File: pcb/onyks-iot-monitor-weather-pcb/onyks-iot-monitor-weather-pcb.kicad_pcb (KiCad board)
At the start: 2 copper layers, 100 x 100 mm, 25 parts, among them J1 53398-0371, J10 Conn_01x02_Pin, J2 53398-0371, J3 53048-0810, J4 53398-0371, J5 53398-0371, J6 53398-0371, J7 53398-0371, J8 53398-0371, J9 53398-0371, Q1 SS8050, Q2 SS8050, U1 ESP32-WROOM-32D, U2 AMS1117, U6 BMP280

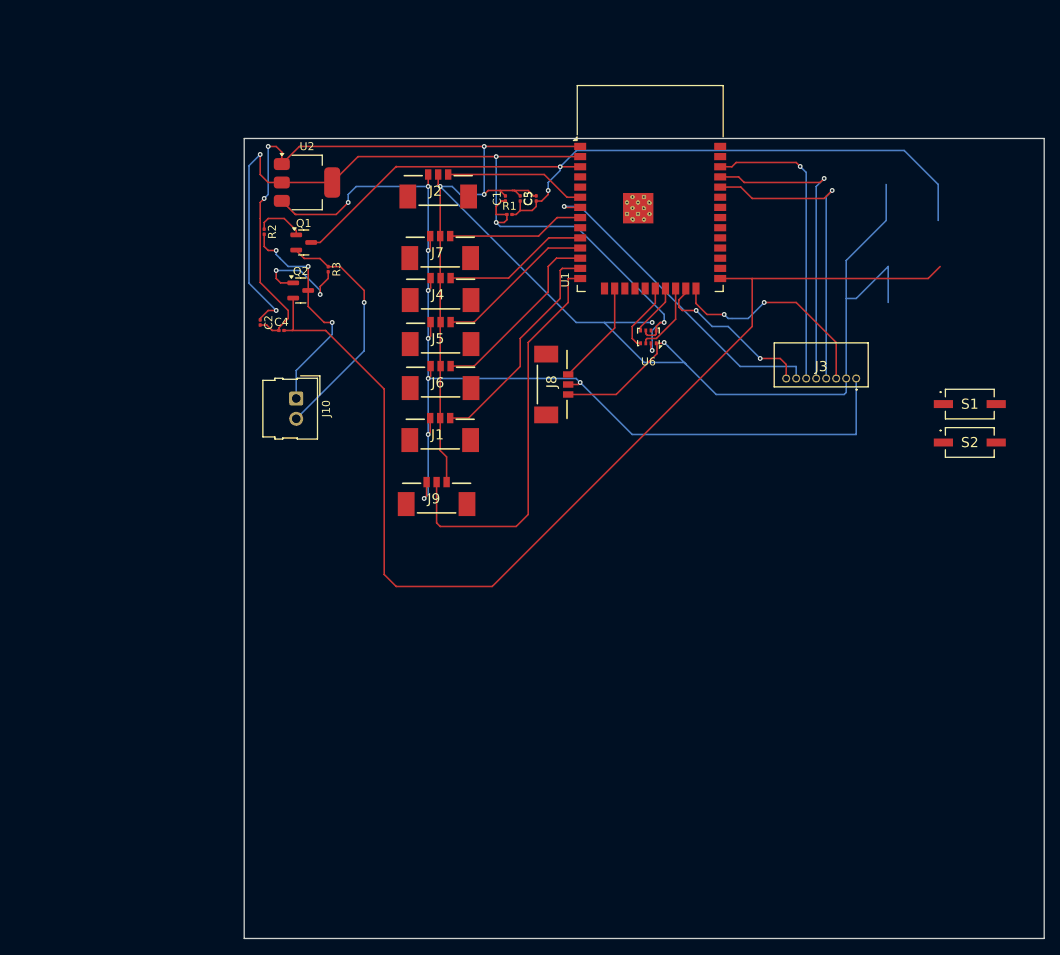
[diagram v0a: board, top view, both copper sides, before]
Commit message: Done my version of PCB
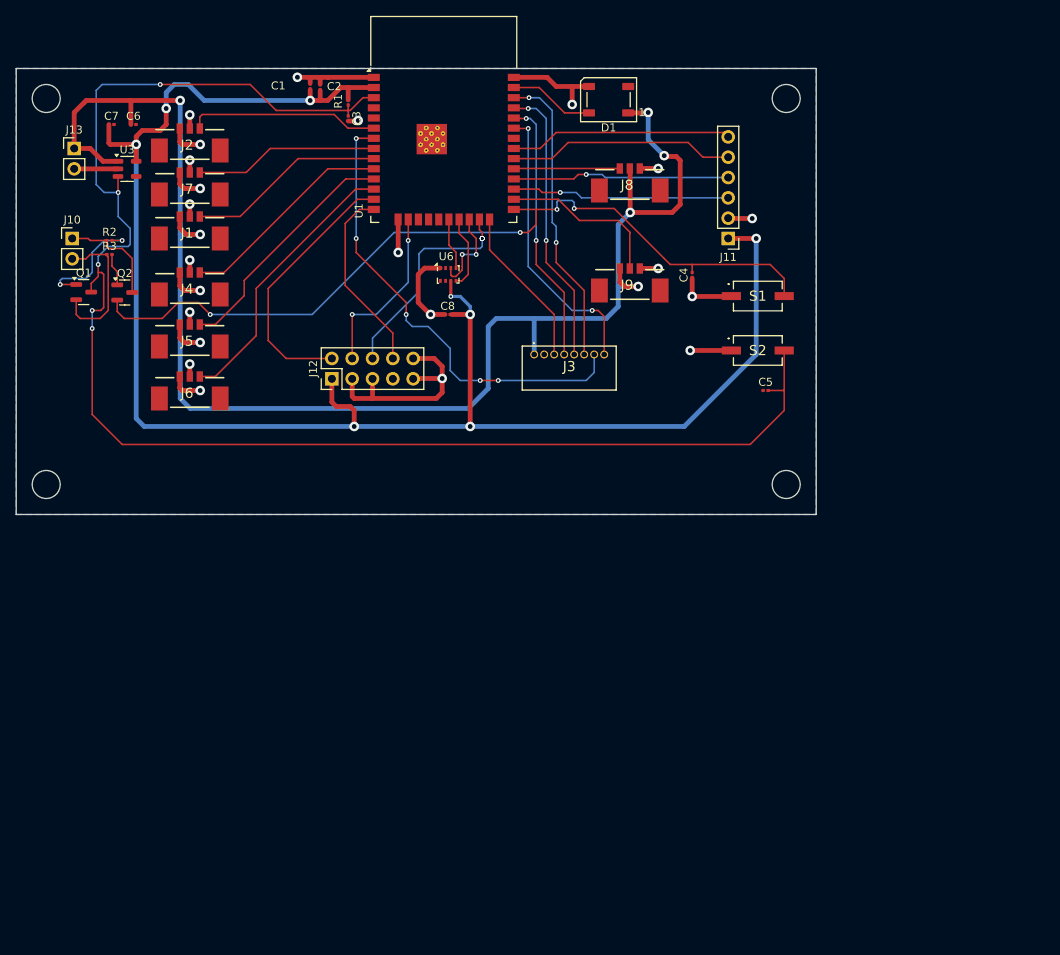
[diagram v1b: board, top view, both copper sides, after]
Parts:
- removed U2: AMS1117, Package_TO_SOT_SMD:SOT-223-3_TabPin2
- added C6: 22uF, Capacitor_SMD:C_0201_0603Metric, F.Cu at (94.7, 54.8)
- added C7: 22uF, Capacitor_SMD:C_0201_0603Metric, F.Cu at (91.9, 54.8)
- added C8: 22uF, Capacitor_SMD:C_0201_0603Metric, F.Cu at (133.9, 78.5)
- added D1: WS2812B, LED_SMD:LED_WS2812B_PLCC4_5.0x5.0mm_P3.2mm, F.Cu at (154.1, 51.6)
- added J11: Conn_01x06_Pin, Connector_PinHeader_2.54mm:PinHeader_1x06_P2.54mm_Vertical, F.Cu at (169.0, 69.0)
- added J12: Conn_02x05_Odd_Even, Connector_PinHeader_2.54mm:PinHeader_2x05_P2.54mm_Vertical, F.Cu at (119.5, 86.5)
- added J13: Conn_01x02_Pin, Connector_PinHeader_2.54mm:PinHeader_1x02_P2.54mm_Vertical, F.Cu at (87.2, 57.8)
- added U3: TLV75733PDBV, Package_TO_SOT_SMD:SOT-23-5, F.Cu at (93.9, 60.3)
- J10: footprint Connector_Molex:Molex_SL_171971-0002_1x02_P2.54mm_Vertical -> Connector_PinHeader_2.54mm:PinHeader_1x02_P2.54mm_Vertical
- moved C4 51.8 mm to (164.5, 73.6), turned to 90 degrees
- moved J3 40.4 mm to (144.8, 83.5), turned to 180 degrees
- moved J1 40.2 mm to (101.7, 66.4)
- moved C5 39.0 mm to (173.7, 88.0), turned to 0 degrees
- moved J9 36.0 mm to (156.7, 72.9)
- moved J10 34.4 mm to (87.0, 69.0), turned to 0 degrees
- moved J7 32.3 mm to (101.7, 60.9)
- moved J2 31.6 mm to (101.7, 55.4)
- moved J6 31.4 mm to (101.7, 86.4)
- moved J4 31.4 mm to (101.7, 73.4)
- moved J5 31.4 mm to (101.7, 79.9)
- moved C2 30.3 mm to (118.0, 50.1), turned to 90 degrees
- moved S1 29.7 mm to (172.7, 76.2)
- moved S2 28.9 mm to (172.7, 83.0)
- moved Q1 28.2 mm to (88.4, 75.7)
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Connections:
- U1 pad 13: /Hall 6 -> /MTMS
- U1 pad 14: /DHT22 -> /MTDI
- U1 pad 16: /SEN0219 -> /MTCK
- U1 pad 23: /PMS_SELECT -> /MTDO
- U1 pad 26: unconnected-(U1-IO4-Pad26) -> /DHT22
- U1 pad 27: unconnected-(U1-IO16-Pad27) -> /UART_PROGRAM_RXD
- U1 pad 28: unconnected-(U1-IO17-Pad28) -> /UART_PROGRAM_TXD
- U1 pad 29: unconnected-(U1-IO5-Pad29) -> /SEN0219
- U1 pad 30: unconnected-(U1-IO18-Pad30) -> /UART_PROGRAM_DTR
- U1 pad 31: unconnected-(U1-IO19-Pad31) -> /UART_PROGRAM_RTS
- U1 pad 33: unconnected-(U1-IO21-Pad33) -> /PMS_SELECT
- U1 pad 37: unconnected-(U1-IO23-Pad37) -> /LED
- U1 pad 9: unconnected-(U1-IO33-Pad9) -> /Hall 6
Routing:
- net GND: track 256.8 -> 100.2 mm, vias 7 -> 17
- net /3V3: track 118.6 -> 213.6 mm, vias 6 -> 8
- net /EN: track 103.2 -> 190.7 mm, vias 2 -> 5
- net VCC: track 138.5 -> 223.2 mm, vias 9 -> 11
- net /MTMS: track 0.00 -> 33.2 mm
- net /IO0: track 137.0 -> 104.7 mm, vias 0 -> 4
- net /DHT22: track 50.8 -> 20.8 mm
- net /UART_PROGRAM_DTR: track 0.00 -> 28.4 mm
- net /UART_PROGRAM_RTS: track 0.00 -> 27.9 mm
- net /MTDO: track 0.00 -> 27.3 mm, vias 0 -> 5
- net /UART_PROGRAM_RXD: track 0.00 -> 27.3 mm, vias 0 -> 1
- net /UART_PROGRAM_TXD: track 0.00 -> 27.2 mm, vias 0 -> 1
- net /MTDI: track 0.00 -> 23.6 mm
- net /MTCK: track 0.00 -> 22.0 mm, vias 0 -> 2
- net /PMS_PWM: track 40.8 -> 58.4 mm, vias 1 -> 5
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- added copper zone on B.Cu, net GND
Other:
- board size 100 x 100 mm -> 100 x 55.8 mm
